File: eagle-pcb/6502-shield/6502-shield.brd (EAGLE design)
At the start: 101.6 x 53.3 mm, 45 parts, among them SW1 MCSLPT4644B1TR-TACT-SW, SW2 PCM12SMTR-SPDT-RIGHT-ANG, SW3 MCSLPT4644B1TR-TACT-SW, U1 AT28C256TSOP-28, U2 W65C02S, U3 AS6C62256, U4 W65C22, U5 MACHXO-FPGA100TQFP

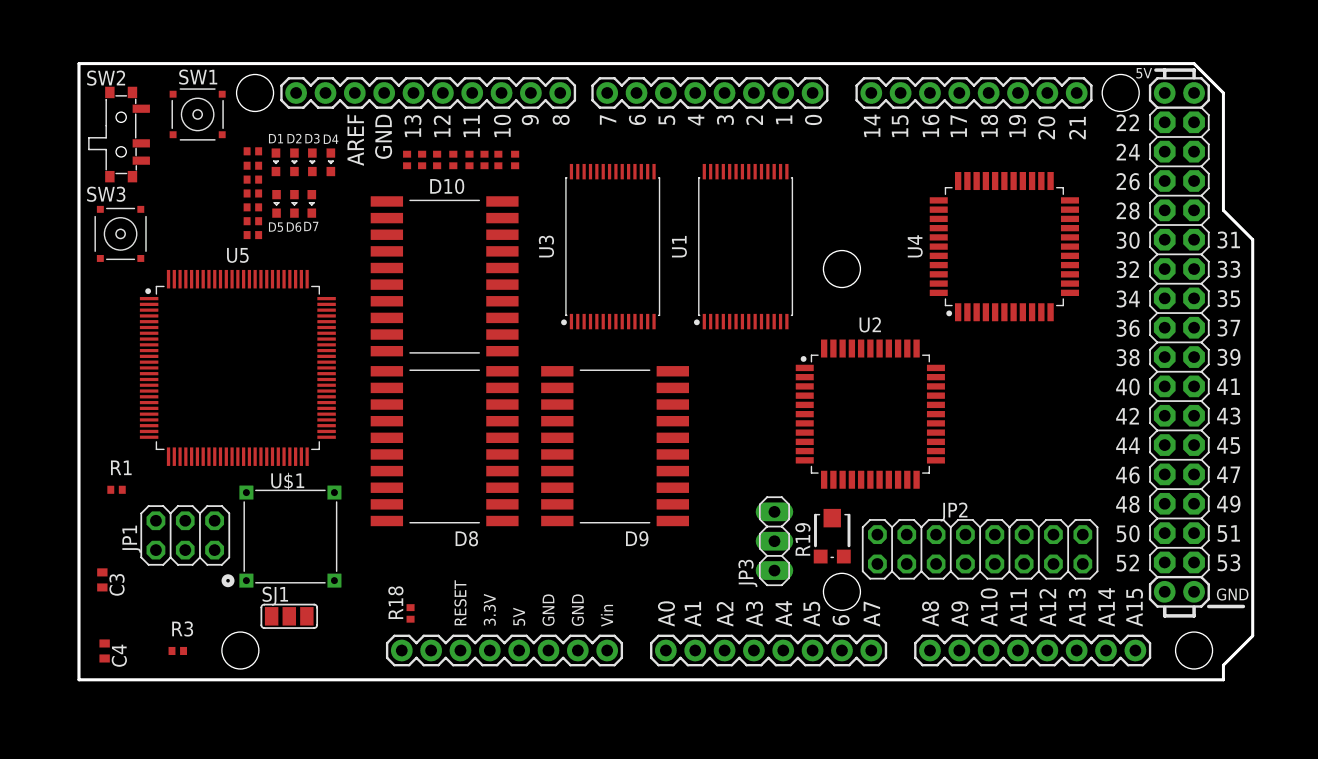
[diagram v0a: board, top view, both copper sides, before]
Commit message: fully routed, getting close
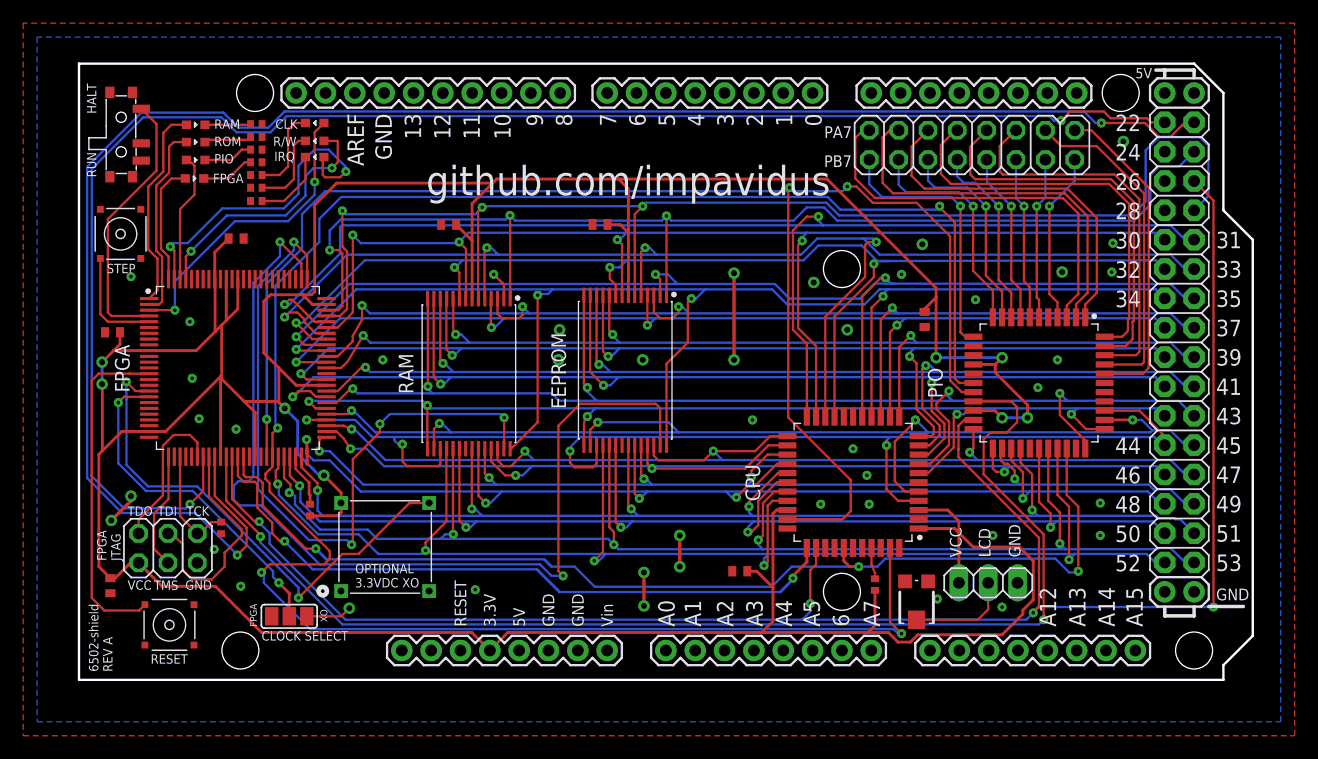
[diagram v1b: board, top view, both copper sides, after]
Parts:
- removed D10, D8, D9: ACDC02-41SGWA-DUAL-7SEG, 6502-shield:ACDC02-41S-DUAL-7SEG
- removed R10, R11, R12, R13, R14, R15, R16, R17: 330, rcl:R0402
- removed SW1: MCSLPT4644B1TR-TACT-SW, 6502-shield:MCSLPT4644B1TR-TACT-SW
- removed U$1: CRYSTAL-OSC-DIP8/4, 6502-shield:DIP8/4
- removed U1: AT28C256TSOP-28, 6502-shield:SOP55P1340X120-28N
- removed U2: W65C02S, 6502-shield:QFP80P1200X1200X160-44N
- removed U3: AS6C62256, 6502-shield:SOP55P1340X120-28N
- removed U4: W65C22, 6502-shield:QFP80P1200X1200X160-44N
- added C1, C2, C5, C6, C7: 0.1uF, rcl:C0402
- added CPU: W65C02S, 6502-shield:QFP80P1200X1200X160-44N
- added EEPROM: AT28C256TSOP-28, 6502-shield:SOP55P1340X120-28N
- added EXT_XO: CRYSTAL-OSC-DIP8/4, 6502-shield:DIP8/4
- added PB_RESET: MCSLPT4644B1TR-TACT-SW, 6502-shield:MCSLPT4644B1TR-TACT-SW
- added PIO: W65C22, 6502-shield:QFP80P1200X1200X160-44N
- added RAM: AS6C62256, 6502-shield:SOP55P1340X120-28N
- D1, D2, D3, D4, D5, D6, D7: value (none) -> RED
- moved R18 40.3 mm to (68.9, 8.25), turned to 270 degrees
- moved JP2 35.0 mm to (77.3, 46.3), turned to 180 degrees
- moved C4 27.6 mm to (2.90, 30.1), turned to 180 degrees
- moved JP3 18.8 mm to (78.7, 8.40), turned to 0 degrees
- moved R1 16.8 mm to (20.0, 14.7), turned to 270 degrees
- moved D4 11.9 mm to (10.0, 43.4), turned to 180 degrees
- moved R3 11.3 mm to (12.3, 13.2), turned to 90 degrees
- moved D3 10.1 mm to (10.1, 45.0), turned to 180 degrees
- moved R19 9.32 mm to (72.5, 6.70), turned to 180 degrees
- moved D2 8.73 mm to (10.1, 46.5), turned to 180 degrees
- moved R2 8.51 mm to (15.3, 47.0)
- moved D5 7.74 mm to (20.4, 48.2), turned to 0 degrees
- moved D1 7.67 mm to (10.1, 48.0), turned to 180 degrees
- moved D6 5.72 mm to (20.4, 46.6), turned to 0 degrees
- moved R7 5.01 mm to (15.3, 45.9), turned to 180 degrees
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- renumbered SJ1 to J1, SW2 to SW_RUNHALT, SW3 to PB_STEP, U5 to FPGA
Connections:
- removed net DIGIT1_EN: D8.18, D8.3, FPGA.87
- removed net DIGIT2_EN: D8.13, D8.8, FPGA.89
- removed net DIGIT3_EN: D9.18, D9.3, FPGA.91
- removed net DIGIT4_EN: D9.13, D9.8, FPGA.94
- removed net DIGIT5_EN: D10.18, D10.3, FPGA.95
- removed net DIGIT6_EN: D10.13, D10.8, FPGA.96
- removed net DIGIT_A: FPGA.78, R10.2
- removed net DIGIT_B: FPGA.79, R11.2
- removed net DIGIT_C: FPGA.80, R12.2
- removed net DIGIT_D: FPGA.81, R13.2
- removed net DIGIT_DP: FPGA.86, R17.2
- removed net DIGIT_E: FPGA.82, R14.2
- removed net DIGIT_F: FPGA.83, R15.2
- removed net DIGIT_G: FPGA.85, R16.2
- removed net N$23: D10.12, D10.17, D8.12, D8.17, D9.12, D9.17, R10.1
- removed net N$24: D10.11, D10.16, D8.11, D8.16, D9.11, D9.16, R11.1
- removed net N$25: D10.4, D10.9, D8.4, D8.9, D9.4, D9.9, R12.1
- removed net N$26: D10.2, D10.7, D8.2, D8.7, D9.2, D9.7, R13.1
- removed net N$27: D10.1, D10.6, D8.1, D8.6, D9.1, D9.6, R14.1
- removed net N$28: D10.14, D10.19, D8.14, D8.19, D9.14, D9.19, R15.1
- removed net N$29: D10.15, D10.20, D8.15, D8.20, D9.15, D9.20, R16.1
- removed net N$30: D10.10, D10.5, D8.10, D8.5, D9.10, D9.5, R17.1
- removed net ROM_PGM: FPGA.34, PCB1.45
- new net EEPROM_PGM: FPGA.34, PCB1.23
- net A0: now also CPU.4, EEPROM.17, PCB1.44, PIO.36, RAM.17; no longer PCB1.22, U1.17, U2.4, U3.17, U4.36
- net A1: now also CPU.5, EEPROM.16, PCB1.45, PIO.35, RAM.16; no longer PCB1.24, U1.16, U2.5, U3.16, U4.35
- net A10: now also CPU.15, EEPROM.28, PCB1.34, RAM.28; no longer PCB1.42, U1.28, U2.15, U3.28
- net A11: now also CPU.16, EEPROM.2, PCB1.35, RAM.2; no longer PCB1.44, U1.2, U2.16, U3.2
- net A12: now also CPU.19, EEPROM.9, PCB1.32, RAM.9; no longer PCB1.46, U1.9, U2.19, U3.9
- net A13: now also CPU.20, EEPROM.5, PCB1.33, RAM.5; no longer PCB1.48, U1.5, U2.20, U3.5
- net A14: now also CPU.21, EEPROM.8, PCB1.30, RAM.8; no longer PCB1.50, U1.8, U2.21, U3.8
- net A15: now also CPU.22, PCB1.31; no longer PCB1.52, U2.22
- net A2: now also CPU.7, EEPROM.15, PCB1.42, PIO.34, RAM.15; no longer PCB1.26, U1.15, U2.7, U3.15, U4.34
- net A3: now also CPU.8, EEPROM.14, PCB1.43, PIO.33, RAM.14; no longer PCB1.28, U1.14, U2.8, U3.14, U4.33
- net A4: now also CPU.9, EEPROM.13, PCB1.40, RAM.13; no longer PCB1.30, U1.13, U2.9, U3.13
- net A5: now also CPU.10, EEPROM.12, PCB1.41, RAM.12; no longer PCB1.32, U1.12, U2.10, U3.12
- net A6: now also CPU.11, EEPROM.11, PCB1.38, RAM.11; no longer PCB1.34, U1.11, U2.11, U3.11
- net A7: now also CPU.12, EEPROM.10, PCB1.39, RAM.10; no longer PCB1.36, U1.10, U2.12, U3.10
- net A8: now also CPU.13, EEPROM.4, PCB1.36, RAM.4; no longer PCB1.38, U1.4, U2.13, U3.4
- net A9: now also CPU.14, EEPROM.3, PCB1.37, RAM.3; no longer PCB1.40, U1.3, U2.14, U3.3
- net BE: now also CPU.34; no longer U2.34
- net CLK: now also CPU.35, PCB1.27, PIO.21; no longer PCB1.43, U2.35, U4.21
- net D0: now also CPU.30, EEPROM.18, PCB1.52, PIO.30, RAM.18; no longer PCB1.23, U1.18, U2.30, U3.18, U4.30
- net D1: now also CPU.29, EEPROM.19, PCB1.53, PIO.29, RAM.19; no longer PCB1.25, U1.19, U2.29, U3.19, U4.29
- net D2: now also CPU.28, EEPROM.20, PCB1.50, PIO.28, RAM.20; no longer PCB1.27, U1.20, U2.28, U3.20, U4.28
- net D3: now also CPU.27, EEPROM.22, PCB1.51, PIO.26, RAM.22; no longer PCB1.29, U1.22, U2.27, U3.22, U4.26
- net D4: now also CPU.26, EEPROM.23, PCB1.48, PIO.25, RAM.23; no longer PCB1.31, U1.23, U2.26, U3.23, U4.25
- net D5: now also CPU.25, EEPROM.24, PCB1.49, PIO.24, RAM.24; no longer PCB1.33, U1.24, U2.25, U3.24, U4.24
- net D6: now also CPU.24, EEPROM.25, PCB1.46, PIO.23, RAM.25; no longer PCB1.35, U1.25, U2.24, U3.25, U4.23
- net D7: now also CPU.23, EEPROM.26, PCB1.47, PIO.22, RAM.26; no longer PCB1.37, U1.26, U2.23, U3.26, U4.22
- net DMA: now also PCB1.22; no longer PCB1.47
- net GND: now also C1.2, C2.2, C5.2, C6.2, C7.2, EEPROM.21, EXT_XO.4, PB_RESET.T2, PIO.39, RAM.21; no longer SW1.T2, U$1.4, U1.21, U3.21, U4.39
- net IO_EN: now also PIO.19; no longer U4.19
- net IRQN: now also CPU.43, PIO.17; no longer U2.43, U4.17
- net N$3: now also PB_RESET.T4; no longer SW1.T4
- net N$31: now also CPU.41; no longer U2.41
- net N$34: now also EXT_XO.5; no longer U$1.5
- net OE: now also EEPROM.1, PCB1.25, RAM.1; no longer PCB1.39, U1.1, U3.1
- net PA0: now also PIO.40; no longer U4.40
- net PA1: now also PIO.41; no longer U4.41
- net PA2: now also PIO.42; no longer U4.42
- net PA3: now also PIO.43; no longer U4.43
- net PA4: now also PIO.44; no longer U4.44
- net PA5: now also PIO.1; no longer U4.1
- net PA6: now also PIO.2; no longer U4.2
- net PA7: now also PIO.3; no longer U4.3
- net PB0: now also PIO.4; no longer U4.4
- net PB1: now also PIO.6; no longer U4.6
- net PB2: now also PIO.7; no longer U4.7
- net PB3: now also PIO.8; no longer U4.8
- net PB4: now also PIO.9; no longer U4.9
- net PB5: now also PIO.10; no longer U4.10
- net PB6: now also PIO.11; no longer U4.11
- net PB7: now also PIO.12; no longer U4.12
- net RAM_EN: now also RAM.27; no longer U3.27
- net RESETN: now also CPU.38, PIO.31; no longer U2.38, U4.31
- net ROM_EN: now also EEPROM.27; no longer U1.27
- net RW: now also CPU.32, PIO.18; no longer U2.32, U4.18
- net VCC: now also C1.1, C2.1, C5.1, C6.1, C7.1, CPU.1, CPU.3, CPU.31, EEPROM.7, EXT_XO.8, PIO.15, PIO.20, RAM.7; no longer U$1.8, U1.7, U2.1, U2.3, U2.31, U3.7, U4.15, U4.20
- net WE: now also EEPROM.6, PCB1.29, RAM.6; no longer PCB1.41, U1.6, U3.6
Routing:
- net VCC: track 0.00 -> 368.6 mm, vias 0 -> 8
- net IRQN: track 0.00 -> 178.4 mm, vias 0 -> 4
- net CLK: track 0.00 -> 159.1 mm, vias 0 -> 4
- net EEPROM_PGM: track 0.00 -> 153.0 mm, vias 0 -> 2
- net DMA: track 0.00 -> 137.7 mm, vias 0 -> 2
- net RW: track 0.00 -> 132.3 mm, vias 0 -> 3
- net A10: track 0.00 -> 123.9 mm, vias 0 -> 4
- net D0: track 0.00 -> 123.1 mm, vias 0 -> 5
- net D1: track 0.00 -> 118.4 mm, vias 0 -> 5
- net A13: track 0.00 -> 117.3 mm, vias 0 -> 4
- net WE: track 0.00 -> 114.5 mm, vias 0 -> 3
- net D2: track 0.00 -> 112.4 mm, vias 0 -> 5
- net A3: track 0.00 -> 111.1 mm, vias 0 -> 5
- net A14: track 0.00 -> 108.8 mm, vias 0 -> 4
- net A15: track 0.00 -> 108.2 mm, vias 0 -> 2
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- added copper zone on layer 1, net GND
- added copper zone on layer 16, net GND
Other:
- board text added: "6502-shield REV A"
- board text added: "CLK"
- board text added: "CLOCK SELECT"
- board text added: "FPGA"
- board text added: "FPGA JTAG"
- board text added: "GND"
- board text added: "HALT"
- board text added: "IRQ"
- board text added: "LCD"
- board text added: "OPTIONAL 3.3VDC XO"
- board text added: "PA7"
- board text added: "PB7"
- board text added: "PIO"
- board text added: "R/W"
- board text added: "RAM"
- board text added: "RESET"
- board text added: "ROM"
- board text added: "RUN"
- board text added: "STEP"
- board text added: "TCK"
- board text added: "TDI"
- board text added: "TDO"
- board text added: "TMS"
- board text added: "VCC"
- board text added: "XO"
- board text added: "github.com/impavidus"
